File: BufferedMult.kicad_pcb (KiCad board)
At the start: 2 copper layers, 20 x 108 mm, 27 parts, among them J1 EURORACK_PWR_10PIN, J2 IN_1, J3 OUT_1A, J4 OUT_1B, J5 OUT_1C, J6 IN_2, J7 OUT_2A, J8 OUT_2B, J9 OUT_2C, U1 TL074H, U2 TL074H

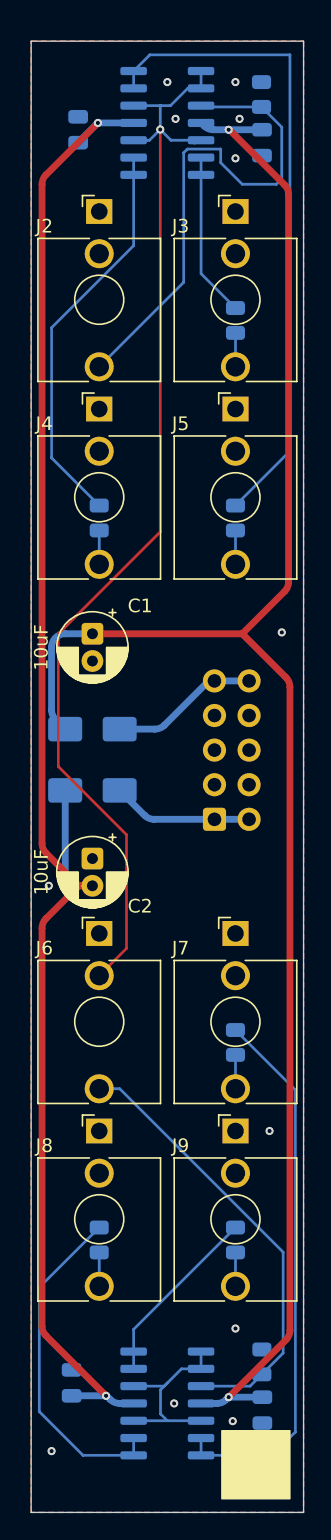
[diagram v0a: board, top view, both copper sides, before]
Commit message: New layout
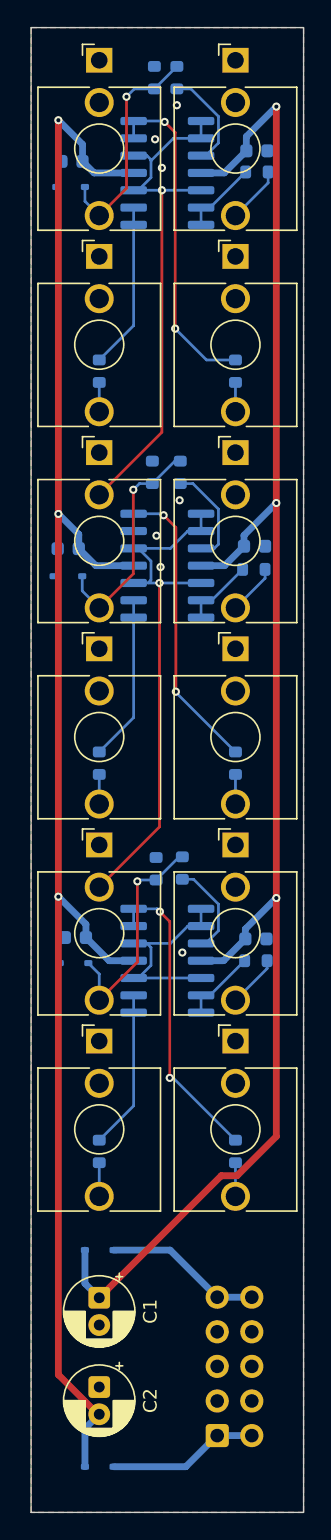
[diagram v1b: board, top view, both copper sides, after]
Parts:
- added C7: 100nF, Capacitor_SMD:C_0603_1608Metric, B.Cu at (36.5, 85.9)
- added C8: 100nF, Capacitor_SMD:C_0603_1608Metric, B.Cu at (23.2, 85.8)
- added D3: PESD12VL1BA, Diode_SMD:D_SOD-323, B.Cu at (22.9, 30.7)
- added D4: PESD12VL1BA, Diode_SMD:D_SOD-323, B.Cu at (22.7, 59.3)
- added D5: PESD12VL1BA, Diode_SMD:D_SOD-323, B.Cu at (23.1, 87.7)
- added J10: IN_3, Connector_Audio:Jack_3.5mm_QingPu_WQP-PJ398SM_Vertical_CircularHoles, F.Cu at (25.0, 79.0)
- added J11: OUT_3A, Connector_Audio:Jack_3.5mm_QingPu_WQP-PJ398SM_Vertical_CircularHoles, F.Cu at (35.0, 79.0)
- added J12: OUT_3B, Connector_Audio:Jack_3.5mm_QingPu_WQP-PJ398SM_Vertical_CircularHoles, F.Cu at (25.0, 93.4)
- added J13: OUT_3C, Connector_Audio:Jack_3.5mm_QingPu_WQP-PJ398SM_Vertical_CircularHoles, F.Cu at (35.0, 93.4)
- added R10: 470R, Resistor_SMD:R_0603_1608Metric, B.Cu at (35.0, 73.0)
- added R11: 100K, Resistor_SMD:R_0603_1608Metric, B.Cu at (29.2, 80.8)
- added R12: 1K, Resistor_SMD:R_0603_1608Metric, B.Cu at (31.1, 80.7)
- added R13: 470R, Resistor_SMD:R_0603_1608Metric, B.Cu at (36.5, 87.5)
- added R14: 470R, Resistor_SMD:R_0603_1608Metric, B.Cu at (25.0, 101.5)
- added R15: 470R, Resistor_SMD:R_0603_1608Metric, B.Cu at (35.0, 101.5)
- added R9: 470R, Resistor_SMD:R_0603_1608Metric, B.Cu at (25.0, 73.0)
- added U3: TL074H, Package_SO:SOIC-14_3.9x8.7mm_P1.27mm, B.Cu at (30.0, 87.5)
- C3, C4, C5, C6: footprint Capacitor_SMD:C_0805_2012Metric -> Capacitor_SMD:C_0603_1608Metric
- D1, D2: value 1N5819 -> 1N5819WS; footprint Diode_SMD:D_SMA -> Diode_SMD:D_SOD-323
- R1, R3, R4, R8: footprint Resistor_SMD:R_0805_2012Metric -> Resistor_SMD:R_0603_1608Metric
- R2, R7: value 470R -> 1K; footprint Resistor_SMD:R_0805_2012Metric -> Resistor_SMD:R_0603_1608Metric
- R5: value 100K -> 470R; footprint Resistor_SMD:R_0805_2012Metric -> Resistor_SMD:R_0603_1608Metric
- R6: value 470R -> 100K; footprint Resistor_SMD:R_0805_2012Metric -> Resistor_SMD:R_0603_1608Metric
- moved R5 72.8 mm to (35.0, 44.2), turned to -90 degrees
- moved C5 63.4 mm to (36.4, 57.1), turned to 0 degrees
- moved U2 61.5 mm to (30.0, 58.5)
- moved C6 61.2 mm to (22.7, 57.2), turned to 0 degrees
- moved R7 56.7 mm to (30.9, 51.6)
- moved D2 49.6 mm to (25.0, 124.6)
- moved R8 49.2 mm to (36.4, 58.8), turned to 0 degrees
- moved C1 48.7 mm to (25.0, 112.2)
- moved J1 45.2 mm to (33.7, 122.4)
- moved R6 42.3 mm to (28.9, 51.6), turned to 90 degrees
- moved C2 38.8 mm to (25.0, 118.8)
- moved D1 38.2 mm to (25.0, 108.7)
- moved J8 35.4 mm to (25.0, 64.6)
- moved J9 35.4 mm to (35.0, 64.6)
- moved J6 35.3 mm to (25.0, 50.2)
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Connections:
- J2 pad T: CH1_IN -> CH1_JACK_IN
- J6 pad T: CH2_IN -> CH2_JACK_IN
- R1 pad 1: CH1_IN -> CH1_JACK_IN
- R2 pad 1: CH1_OP_A -> CH1_JACK_IN
- R2 pad 2: CH1_OUT_A -> CH1_IN
- R3 pad 1: CH1_OP_B -> CH1_OP_A
- R3 pad 2: CH1_OUT_B -> CH1_OUT_A
- R4 pad 1: CH1_OP_C -> CH1_OP_B
- R4 pad 2: CH1_OUT_C -> CH1_OUT_B
- R5 pad 1: CH2_IN -> CH1_OP_C
- R5 pad 2: GND -> CH1_OUT_C
- R6 pad 1: CH2_OP_A -> CH2_JACK_IN
- R6 pad 2: CH2_OUT_A -> GND
- R7 pad 1: CH2_OP_B -> CH2_JACK_IN
- R7 pad 2: CH2_OUT_B -> CH2_IN
- R8 pad 1: CH2_OP_C -> CH2_OP_A
- R8 pad 2: CH2_OUT_C -> CH2_OUT_A
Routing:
- net CH1_BUF: track 83.8 -> 39.2 mm
- net CH2_OP_A: track 40.2 -> 5.26 mm
- net CH1_IN: track 37.8 -> 7.50 mm
- net CH2_IN: track 32.9 -> 7.56 mm
- net CH1_OP_C: track 48.0 -> 24.4 mm, vias 0 -> 2
- net CH2_BUF: track 14.9 -> 38.2 mm, vias 0 -> 1
- net CH3_OP_C: track 0.00 -> 22.5 mm, vias 0 -> 2
- net CH1_OP_B: track 29.5 -> 12.2 mm
- net CH3_JACK_IN: track 0.00 -> 17.0 mm, vias 0 -> 1
- net CH2_JACK_IN: track 0.00 -> 16.9 mm, vias 0 -> 1
- net CH1_JACK_IN: track 0.00 -> 16.7 mm, vias 0 -> 1
- net CH3_BUF: track 0.00 -> 16.1 mm
- net CH2_OP_B: track 24.9 -> 12.2 mm
- net CH3_OP_B: track 0.00 -> 11.7 mm
- net CH2_OP_C: track 13.5 -> 23.1 mm, vias 0 -> 2
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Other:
- board size 20 x 108 mm -> 20 x 109 mm
- board text removed: "-12V"
- board text removed: "Version: 1.1"
- board text removed: "github.com/domesticmouse/BufferedMult-SKiDL"
